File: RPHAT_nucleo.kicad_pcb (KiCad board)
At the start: 2 copper layers, 24 parts, among them J1 Raspberry_Pi_2_3, J2 Conn_01x04_Female, J3 Conn_01x04_Female, J4 Conn_01x04_Female, U1 NUCLEO-F446RE, U2 MCP2551-I-SN, U3 MCP2515-xST, U4 MCP2551-I-SN, U5 MCP2551-I-SN, Y1 Crystal

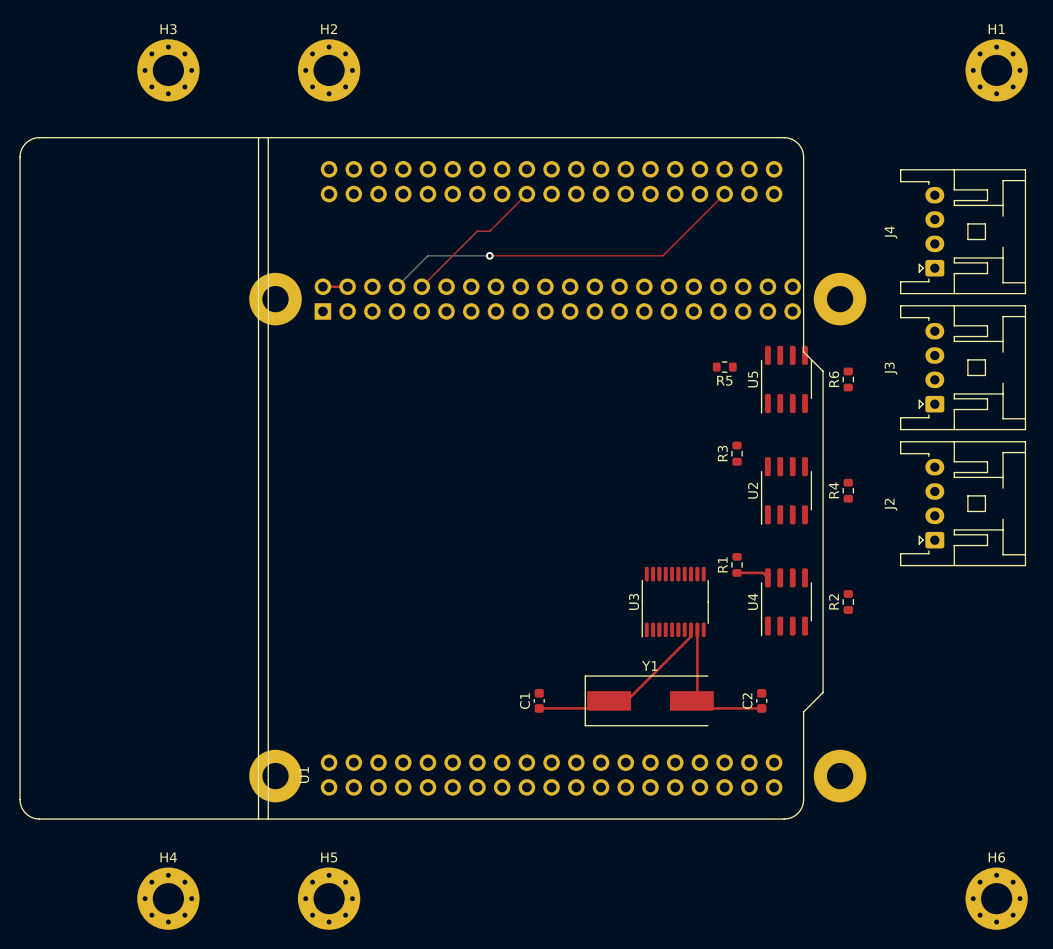
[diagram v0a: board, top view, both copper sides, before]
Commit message: complete
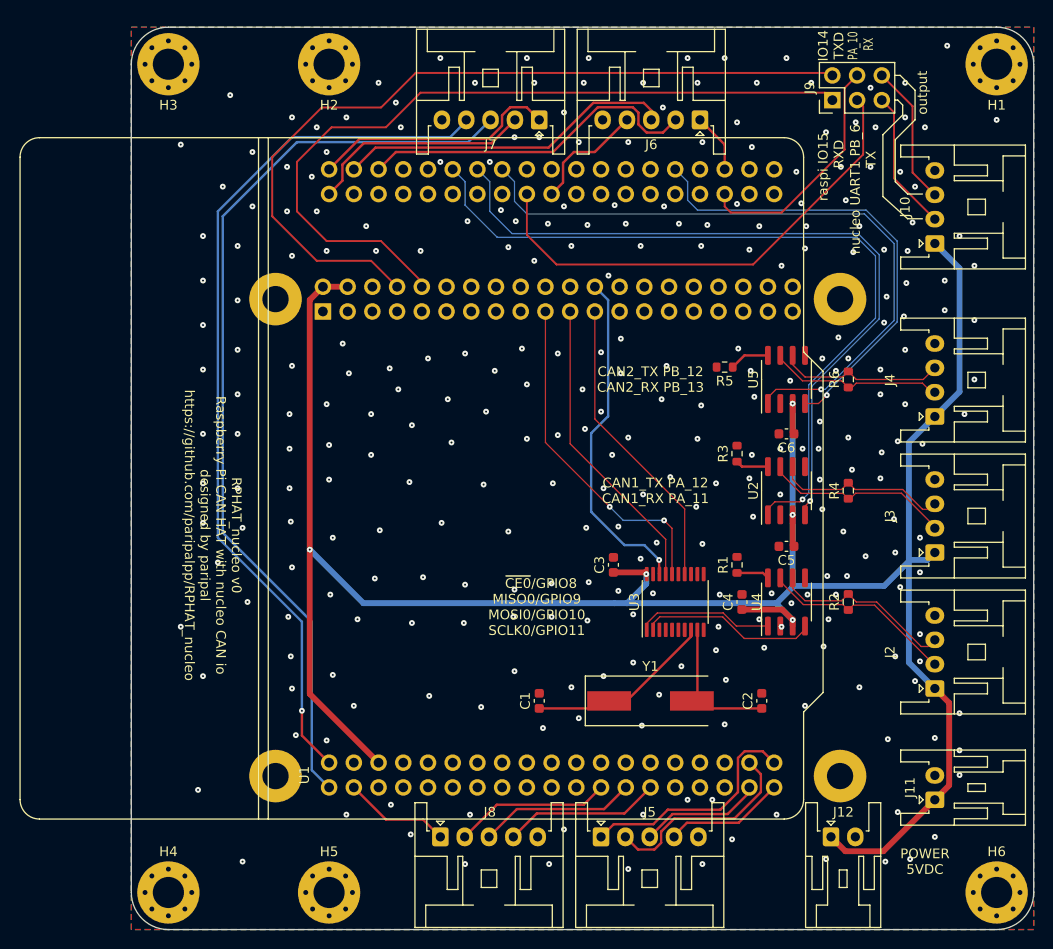
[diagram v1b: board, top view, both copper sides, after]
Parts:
- added C3: 0.1u, Capacitor_SMD:C_0603_1608Metric, F.Cu at (147.3, 105.4)
- added C4: 0.1u, Capacitor_SMD:C_0603_1608Metric, F.Cu at (160.5, 109.2)
- added C5: 0.1u, Capacitor_SMD:C_0603_1608Metric, F.Cu at (165.1, 103.5)
- added C6: 0.1u, Capacitor_SMD:C_0603_1608Metric, F.Cu at (165.1, 91.9)
- added J10: Conn_01x04_Female, Connector_JST:JST_XA_S04B-XASK-1_1x04_P2.50mm_Horizontal, F.Cu at (180.3, 72.4)
- added J11: Conn_01x02_Female, Connector_JST:JST_XA_S02B-XASK-1_1x02_P2.50mm_Horizontal, F.Cu at (180.3, 129.5)
- added J12: Conn_01x02_Female, Connector_JST:JST_XA_S02B-XASK-1_1x02_P2.50mm_Horizontal, F.Cu at (169.7, 133.3)
- added J5: Conn_01x05_Female, Connector_JST:JST_XA_S05B-XASK-1_1x05_P2.50mm_Horizontal, F.Cu at (146.1, 133.3)
- added J6: Conn_01x05_Female, Connector_JST:JST_XA_S05B-XASK-1_1x05_P2.50mm_Horizontal, F.Cu at (156.2, 59.7)
- added J7: Conn_01x05_Female, Connector_JST:JST_XA_S05B-XASK-1_1x05_P2.50mm_Horizontal, F.Cu at (139.7, 59.7)
- added J8: Conn_01x05_Female, Connector_JST:JST_XA_S05B-XASK-1_1x05_P2.50mm_Horizontal, F.Cu at (129.5, 133.3)
- added J9: Conn_02x03_Odd_Even, Connector_PinHeader_2.54mm:PinHeader_2x03_P2.54mm_Vertical, F.Cu at (169.8, 57.7)
- moved J2 15.2 mm to (180.3, 118.1)
- moved J3 15.2 mm to (180.3, 104.1)
- moved J4 15.2 mm to (180.3, 90.2)
- moved H1 0.63 mm to (186.7, 54.0), turned to 180 degrees
- moved H2 0.63 mm to (118.1, 54.0), turned to 180 degrees
- moved H3 0.63 mm to (101.6, 54.0), turned to 180 degrees
- moved H4 0.63 mm to (101.6, 139.1)
- moved H5 0.63 mm to (118.1, 139.1)
- moved H6 0.63 mm to (186.7, 139.1)
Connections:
- J1 pad 1: +3V3 -> unconnected-(J1-Pad1)
- J1 pad 10: /Serial_nu_to_rp -> /UART_RX_rp
- J1 pad 17: +3V3 -> unconnected-(J1-Pad17)
- J1 pad 8: /Serial_rp_to_nu -> /UART_TX_rp
- U1 pad 1: unconnected-(U1-Pad1) -> /nu_PC_10
- U1 pad 2: unconnected-(U1-Pad2) -> /nu_PC_11
- U1 pad 23: unconnected-(U1-Pad23) -> /nu_PC_13
- U1 pad 25: unconnected-(U1-Pad25) -> /nu_PC_14
- U1 pad 27: unconnected-(U1-Pad27) -> /nu_PC_15
- U1 pad 3: unconnected-(U1-Pad3) -> /nu_PC_12
- U1 pad 35: unconnected-(U1-Pad35) -> /nu_PC_2
- U1 pad 36: unconnected-(U1-Pad36) -> /nu_PC_1
- U1 pad 37: unconnected-(U1-Pad37) -> /nu_PC_3
- U1 pad 38: unconnected-(U1-Pad38) -> /nu_PC_0
- U1 pad 39: unconnected-(U1-Pad39) -> /nu_PC_9
- U1 pad 40: unconnected-(U1-Pad40) -> /nu_PC_8
- U1 pad 42: unconnected-(U1-Pad42) -> /nu_PC_6
- U1 pad 44: unconnected-(U1-Pad44) -> /nu_PC_5
- U1 pad 55: /Serial_nu_to_rp -> /UART_TX_nu
- U1 pad 57: unconnected-(U1-Pad57) -> /nu_PC_7
- U1 pad 71: /Serial_rp_to_nu -> /UART_RX_nu
- U1 pad 72: unconnected-(U1-Pad72) -> /nu_PC_4
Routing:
- net +5V: track 2.54 -> 240.8 mm, vias 0 -> 5
- net /nu_PC_10: track 0.00 -> 94.8 mm
- net /nu_PC_11: track 0.00 -> 90.9 mm, vias 0 -> 1
- net /UART_TX_rp: track 0.00 -> 83.2 mm
- net /nuCAN1_TX: track 0.00 -> 81.2 mm, vias 0 -> 1
- net /UART_RX_rp: track 0.00 -> 79.7 mm
- net /nuCAN1_RX: track 0.00 -> 76.6 mm, vias 0 -> 1
- net /nuCAN2_TX: track 0.00 -> 69.4 mm, vias 0 -> 1
- net /UART_TX_nu: track 0.00 -> 50.5 mm
- net /nuCAN2_RX: track 0.00 -> 48.4 mm, vias 0 -> 1
- net /Serial_rp_to_nu: track 37.6 -> 0.00 mm, vias 1 -> 0
- net /nu_PC_5: track 0.00 -> 35.5 mm
- net /rp_~{CS}_MCP2512: track 0.00 -> 34.9 mm, vias 0 -> 1
- net /rp_MOSI: track 0.00 -> 34.8 mm, vias 0 -> 2
- net /nu_PC_6: track 0.00 -> 34.7 mm
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- added copper zone on B.Cu, net GND
- added copper zone on F.Cu, net GND
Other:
- board outline added: 92.7 x 92.7 mm
- board text added: "CAN1_TX PA_12 CAN1_RX PA_11"
- board text added: "CAN2_TX PB_12 CAN2_RX PB_13"
- board text added: "GND PC_11 PC_10 PC_9 PC_8"
- board text added: "GND PC_7 PC_6 PC_5 PC_4"
- board text added: "IO14 TXD"
- board text added: "PA_10 RX"
- board text added: "PC_0 PC_1 PC_2 PC_3 GND"
- board text added: "PC_12 PC_13 PC_14 PC_15 GND"
- board text added: "POWER 5VDC"
- board text added: "RPHAT_nucleo v0 Raspberry Pi CAN HAT with nucleo CAN io designed by paripal https://github.com/paripalpp/RPHAT_nucleo"
- board text added: "nucleo UART1 PB_6 TX"
- board text added: "output"
- board text added: "raspi IO15 RXD"
- board text added: "~{CE0}/GPIO8 MISO0/GPIO9 MOSI0/GPIO10 SCLK0/GPIO11"
